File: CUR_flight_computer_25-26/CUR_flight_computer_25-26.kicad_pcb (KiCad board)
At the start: 4 copper layers, 48.8 x 84.8 mm, 145 parts, among them J1 3220-14-0100-00, J10 PYRO, J11 PYRO, J12 USB_C_Receptacle_USB2.0_16P, J13 Conn_01x04_Pin, J14 Conn_Coaxial_Small, J2 Screw_Terminal_01x02, J3 Screw_Terminal_01x02, J4 XT30PW-M, J5 XT30PW-M, J6 Micro_SD_Card, J7 Conn_01x02_Pin, J8 PYRO, J9 PYRO, Q1 NTR4003N, SW1 GSPTS0018, SW2 SW_SPDT, SW3 GSPTS0018, SW4 GSPTS0018, SW5 GSPTS0018, U1 STM32H523VETx, U10 W25Q32JVSS, U11 SAM-M8Q, U12 BUK9K25-40RAX, U13 BUK9K25-40RAX, U14 USBLC6-2SC6, U2 IIS2MDC, U3 LPS22HB, U4 LSM6DSV80X, U5 E22-400M30S, U6 BU33SD5, U7 LM66200, U8 ZXCT180A4W5, U9 ZXCT180A4W5, Y1 16M18PX/XT324-10/10

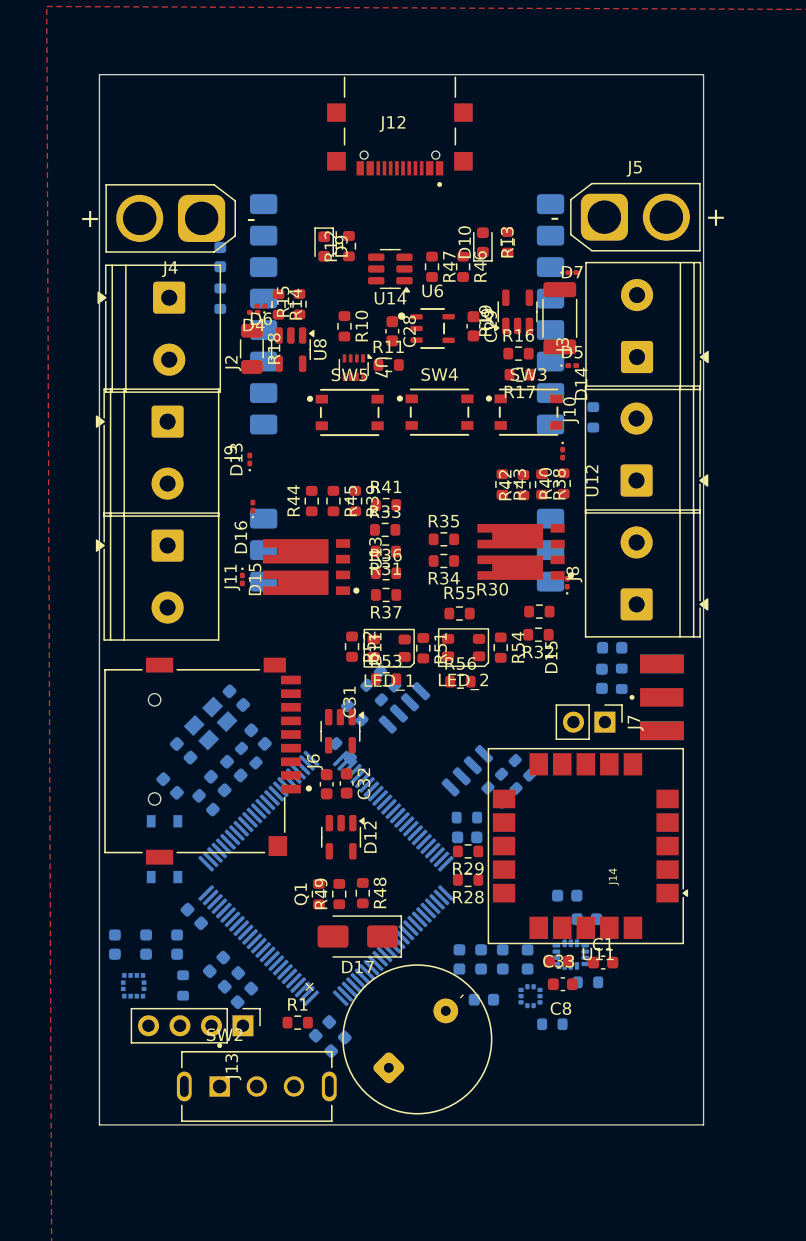
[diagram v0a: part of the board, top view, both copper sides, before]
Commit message: routing updates
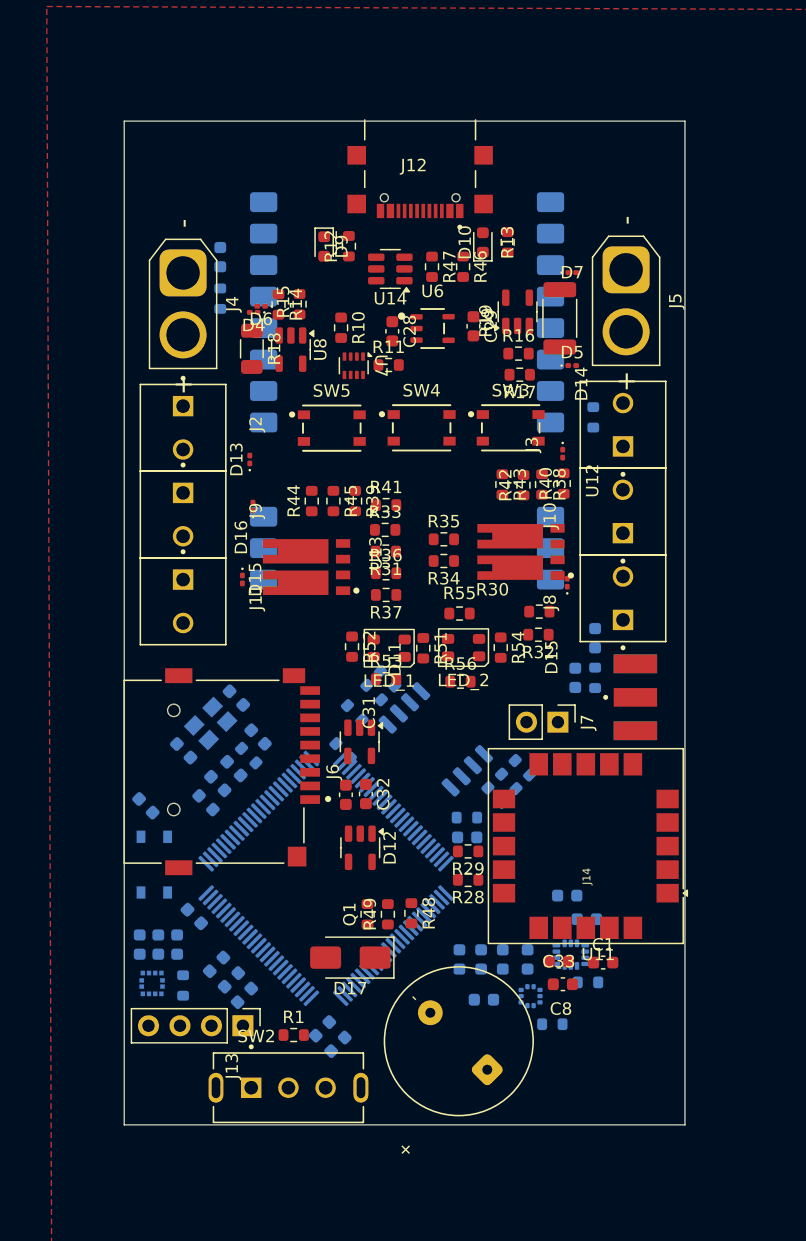
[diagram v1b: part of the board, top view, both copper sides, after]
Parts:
- J10, J11, J2, J3, J8, J9: footprint TerminalBlock_Phoenix:TerminalBlock_Phoenix_PT-1,5-2-5.0-H_1x02_P5.00mm_Horizontal -> Terminal_SAMESKY_TB0011-350-02GR:SAMESKY_TB0011-350-02GR
- moved J2 10.6 mm to (51.0, 60.2)
- moved J9 7.60 mm to (51.0, 67.2)
- moved J3 5.58 mm to (86.5, 60.0)
- moved J11 4.67 mm to (51.0, 74.2)
- moved J4 4.65 mm to (51.0, 47.8), turned to -90 degrees
- moved J5 4.60 mm to (86.8, 47.5), turned to -90 degrees
- moved Q1 4.25 mm to (65.9, 99.5)
- moved R49 4.25 mm to (67.5, 99.5)
- moved R48 4.25 mm to (69.4, 99.4)
- moved J12 3.81 mm to (70.1, 39.1)
- moved J7 3.79 mm to (81.2, 84.0)
- moved R50 3.35 mm to (73.2, 109.8), turned to 135 degrees
- moved J10 2.73 mm to (86.5, 67.0)
- moved SW2 2.55 mm to (59.5, 113.5)
- moved C5 2.52 mm to (48.0, 90.8)
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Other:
- board size 48.8 x 84.8 mm -> 45.2 x 81 mm
